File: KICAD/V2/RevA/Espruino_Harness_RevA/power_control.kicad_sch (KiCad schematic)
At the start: 17 parts, among them J1001 OPERATING_MODE, Q1 2N7002, U1001 TPS2116DRL, U1002 TPS22917DBV

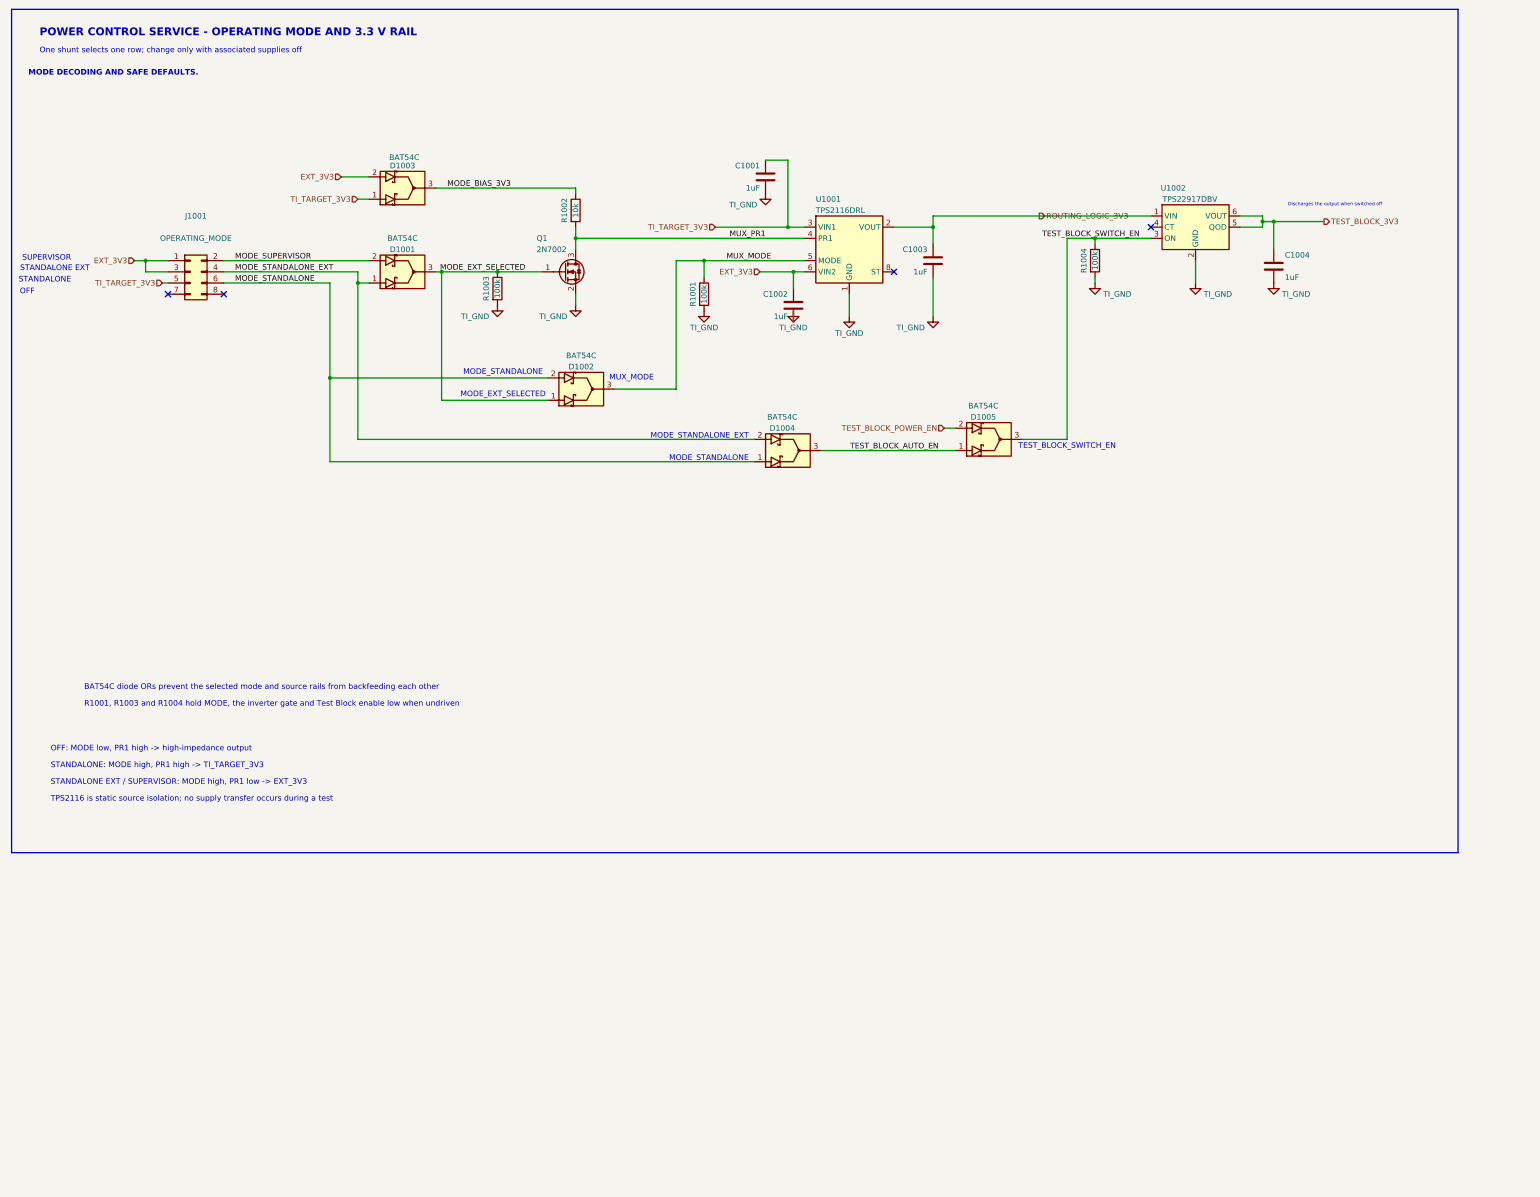
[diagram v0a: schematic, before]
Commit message: Establish Rev-A schematic verification framework
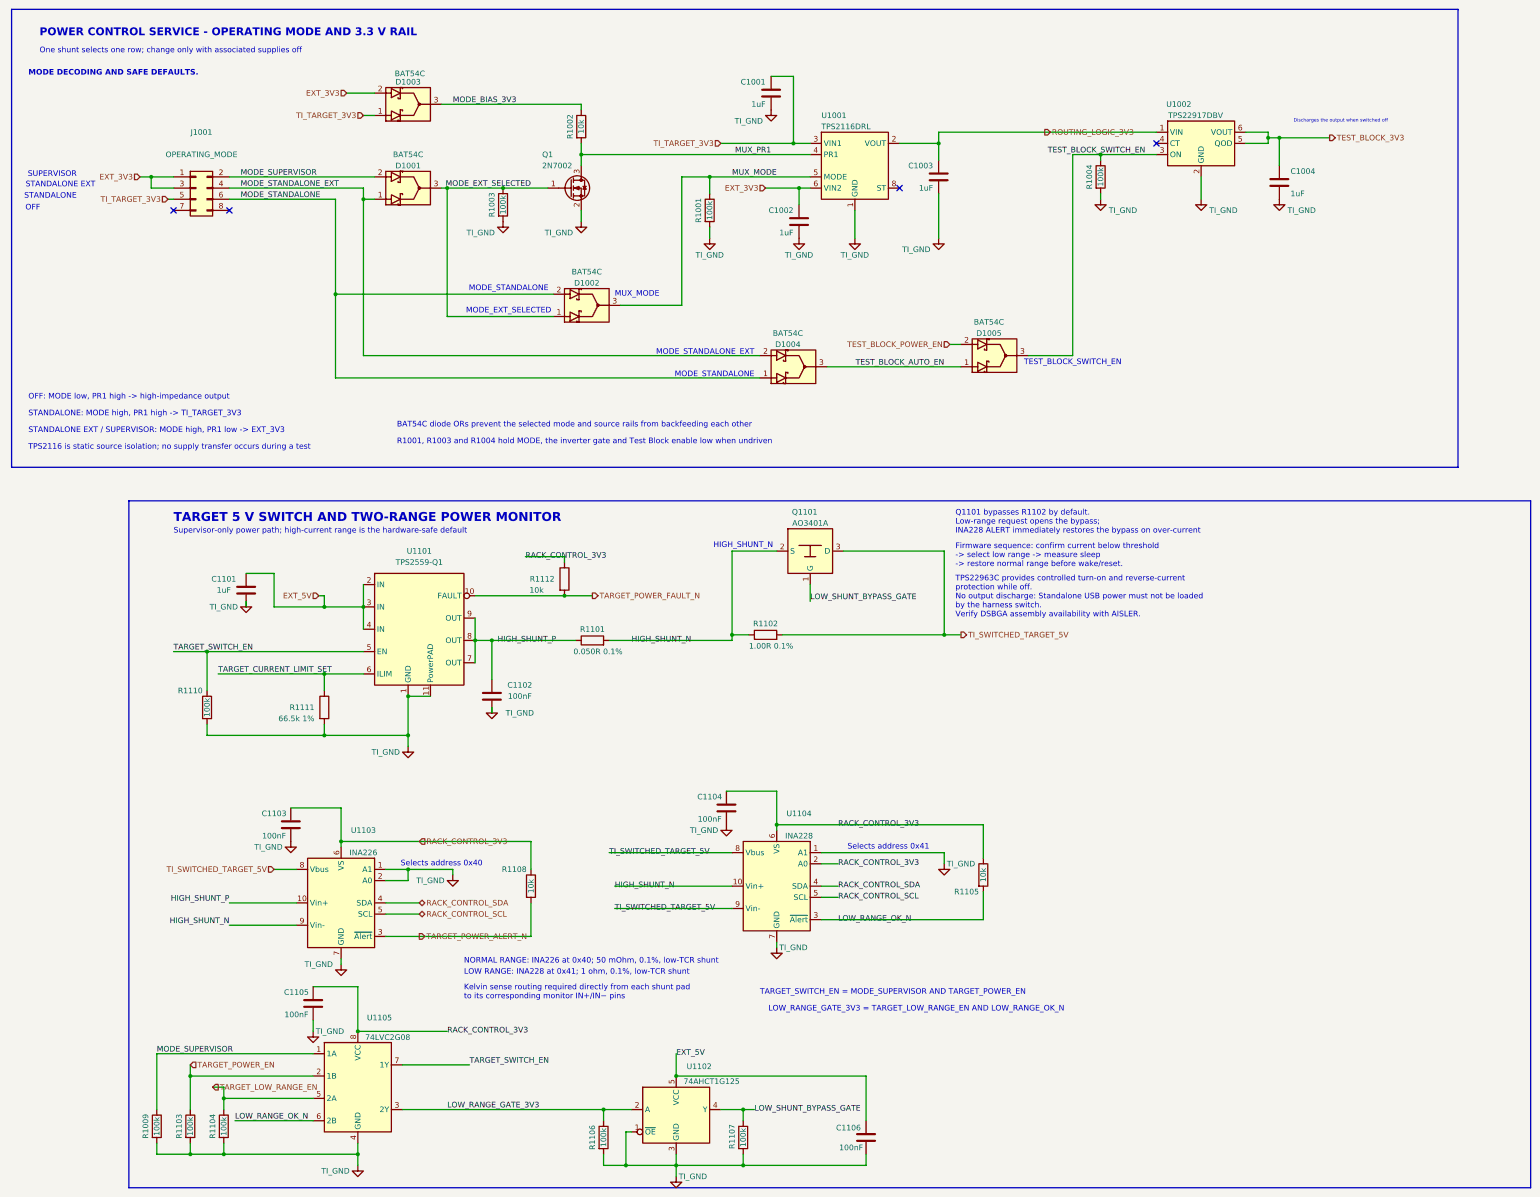
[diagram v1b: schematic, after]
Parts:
- added C1101: 1uF, Capacitor_SMD:C_0603_1608Metric, symbol Espruino_Harness_RevA:C
- added C1102, C1103, C1104, C1105, C1106: 100nF, Capacitor_SMD:C_0603_1608Metric, symbol Espruino_Harness_RevA:C
- added Q1101: AO3401A, Package_TO_SOT_SMD:SOT-23, symbol Espruino_Harness_RevA:AO3401A_LOW_RANGE_BYPASS
- added R1009, R1103, R1104, R1106, R1107, R1110: 100k, Resistor_SMD:R_0603_1608Metric, symbol Espruino_Harness_RevA:R
- added R1101: 0.050R 0.1%, Resistor_SMD:R_0603_1608Metric, symbol Espruino_Harness_RevA:R
- added R1102: 1.00R 0.1%, Resistor_SMD:R_0603_1608Metric, symbol Espruino_Harness_RevA:R
- added R1105, R1108, R1112: 10k, Resistor_SMD:R_0603_1608Metric, symbol Espruino_Harness_RevA:R
- added R1111: 66.5k 1%, Resistor_SMD:R_0603_1608Metric, symbol Espruino_Harness_RevA:R
- added U1101: TPS2559-Q1, symbol Espruino_Harness_RevA:TPS2559Q1_TARGET_POWER_SWITCH
- added U1102: 74AHCT1G125, Package_TO_SOT_SMD:SOT-23-5, symbol Espruino_Harness_RevA:74AHCT1G125_RANGE_DRIVER
- added U1103: INA226, Package_SO:VSSOP-10_3x3mm_P0.5mm, symbol Espruino_Harness_RevA:INA226_HIGH_RANGE
- added U1104: INA228, Package_SO:VSSOP-10_3x3mm_P0.5mm, symbol Espruino_Harness_RevA:INA228_LOW_RANGE
- added U1105: 74LVC2G08, Package_SO:VSSOP-8_2.3x2mm_P0.5mm, symbol Espruino_Harness_RevA:74LVC2G08_POWER_CONTROL
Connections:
- net MODE_SUPERVISOR: now also R1009.1, U1105.1 (1A)
- net TI_GND: now also C1101.2, C1102.2, C1103.2, C1104.2, C1105.2, C1106.2, R1009.2, R1103.2, R1104.2, R1106.2, R1107.2, R1110.2, R1111.2, U1101.1 (GND), U1101.11 (PowerPAD), U1102.1 (~{OE}), U1102.3 (GND), U1103.1 (A1), U1103.2 (A0), U1103.7 (GND), U1104.1 (A1), U1104.7 (GND), U1105.4 (GND)
- new net EXT_5V: C1101.1, C1106.1, U1101.2 (IN), U1101.3 (IN), U1101.4 (IN), U1102.5 (VCC)
- new net HIGH_SHUNT_N: Q1101.2 (S), R1101.2, R1102.1, U1103.9 (Vin-), U1104.10 (Vin+)
- new net HIGH_SHUNT_P: C1102.1, R1101.1, U1101.7 (OUT), U1101.8 (OUT), U1101.9 (OUT), U1103.10 (Vin+)
- new net LOW_RANGE_GATE_3V3: R1106.1, U1102.2 (A), U1105.3 (2Y)
- new net LOW_RANGE_OK_N: R1105.2, U1104.3 (~{Alert}), U1105.6 (2B)
- new net LOW_SHUNT_BYPASS_GATE: Q1101.1 (G), R1107.1, U1102.4 (Y)
- new net RACK_CONTROL_3V3: C1103.1, C1104.1, C1105.1, R1105.1, R1108.1, R1112.1, U1103.6 (VS), U1104.2 (A0), U1104.6 (VS), U1105.8 (VCC)
- new net RACK_CONTROL_SCL: U1103.5 (SCL), U1104.5 (SCL)
- new net RACK_CONTROL_SDA: U1103.4 (SDA), U1104.4 (SDA)
- new net TARGET_CURRENT_LIMIT_SET: R1111.1, U1101.6 (ILIM)
- new net TARGET_LOW_RANGE_EN: R1104.1, U1105.5 (2A)
- new net TARGET_POWER_ALERT_N: R1108.2, U1103.3 (~{Alert})
- new net TARGET_POWER_EN: R1103.1, U1105.2 (1B)
- new net TARGET_POWER_FAULT_N: R1112.2, U1101.10 (FAULT)
- new net TARGET_SWITCH_EN: R1110.1, U1101.5 (EN), U1105.7 (1Y)
- new net TI_SWITCHED_TARGET_5V: Q1101.3 (D), R1102.2, U1103.8 (Vbus), U1104.8 (Vbus), U1104.9 (Vin-)
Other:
- note added: "Firmware sequence: confirm current below threshold -> select low range -> measure sleep -> restore normal range before wake/reset."
- note added: "HIGH_SHUNT_N"
- note added: "Kelvin sense routing required directly from each shunt pad to its corresponding monitor IN+/IN− pins"
- note added: "LOW RANGE: INA228 at 0x41; 1 ohm, 0.1%, low-TCR shunt"
- note added: "LOW_RANGE_GATE_3V3 = TARGET_LOW_RANGE_EN AND LOW_RANGE_OK_N"
- note added: "NORMAL RANGE: INA226 at 0x40; 50 mOhm, 0.1%, low-TCR shunt"
- note added: "Q1101 bypasses R1102 by default. Low-range request opens the bypass; INA228 ALERT immediately restores the bypass on over-current"
- note added: "Selects address 0x40"
- note added: "Selects address 0x41"
- note added: "Supervisor-only power path; high-current range is the hardware-safe default"
- note added: "TARGET 5 V SWITCH AND TWO-RANGE POWER MONITOR"
- note added: "TARGET_SWITCH_EN = MODE_SUPERVISOR AND TARGET_POWER_EN"
- note added: "TPS22963C provides controlled turn-on and reverse-current protection while off. No output discharge: Standalone USB power must not be loaded by the harness switch. Verify DSBGA assembly availability with AISLER."
- moved on the sheet: C1001, C1002, C1003, C1004, D1001, D1002, D1003, D1004, D1005, J1001, Q1, R1001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
